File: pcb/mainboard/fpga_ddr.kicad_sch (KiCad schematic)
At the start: 33 parts, among them U12 MT41K64M16TW, U5 XC6SLX16-FTG256

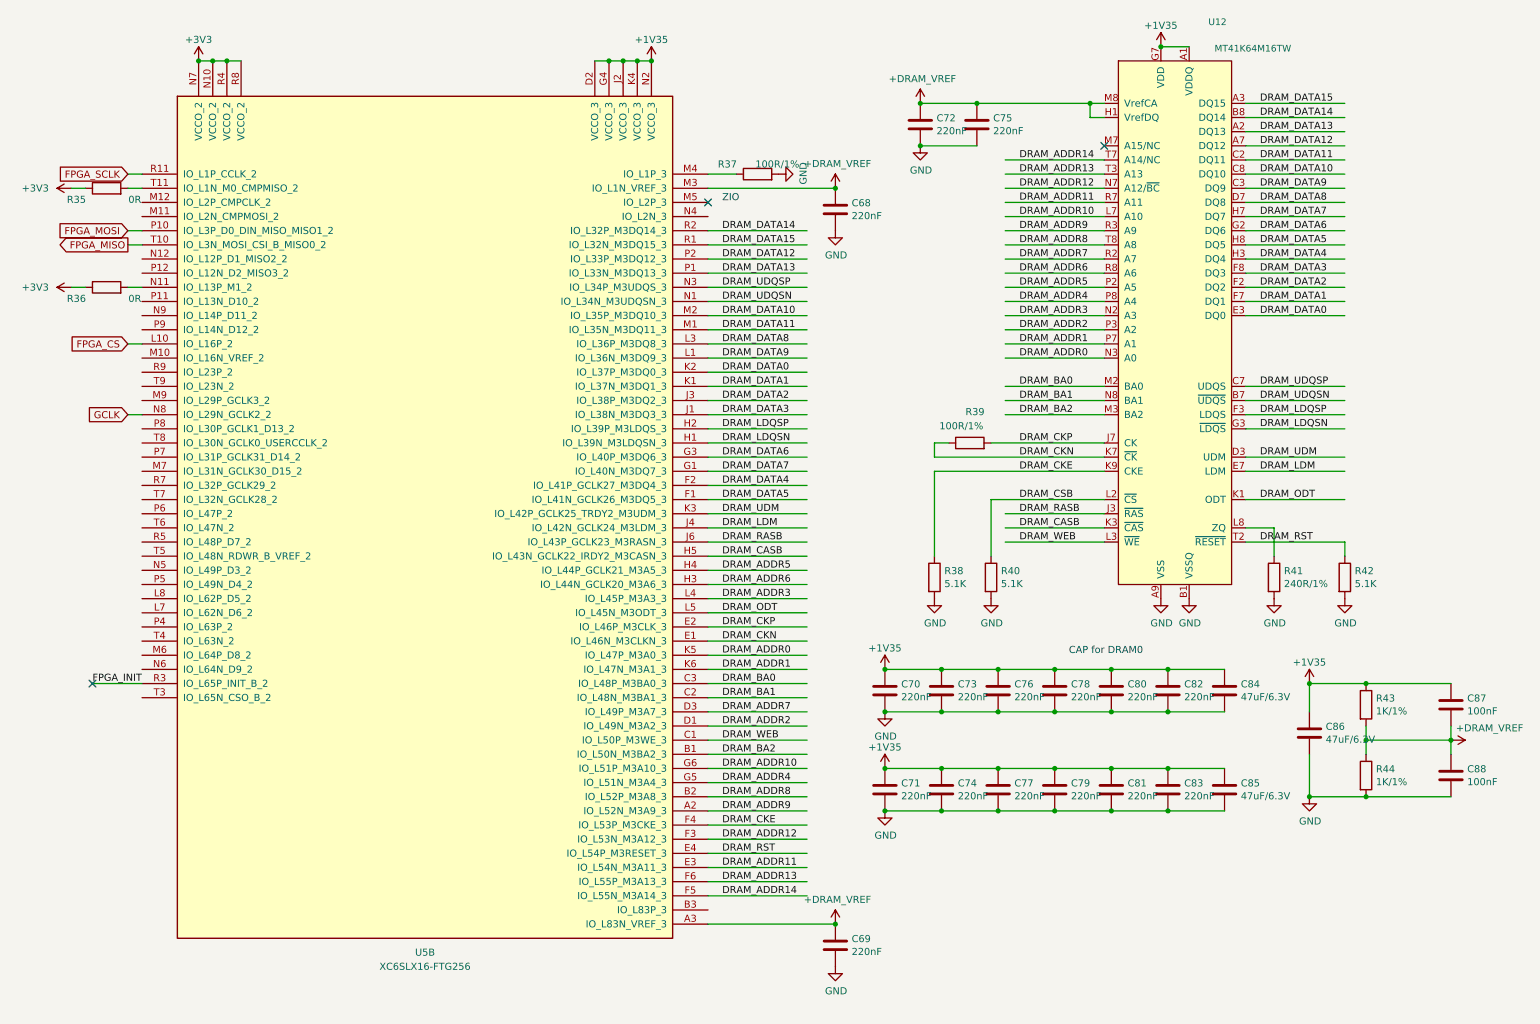
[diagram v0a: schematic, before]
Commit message: PCB r0p9
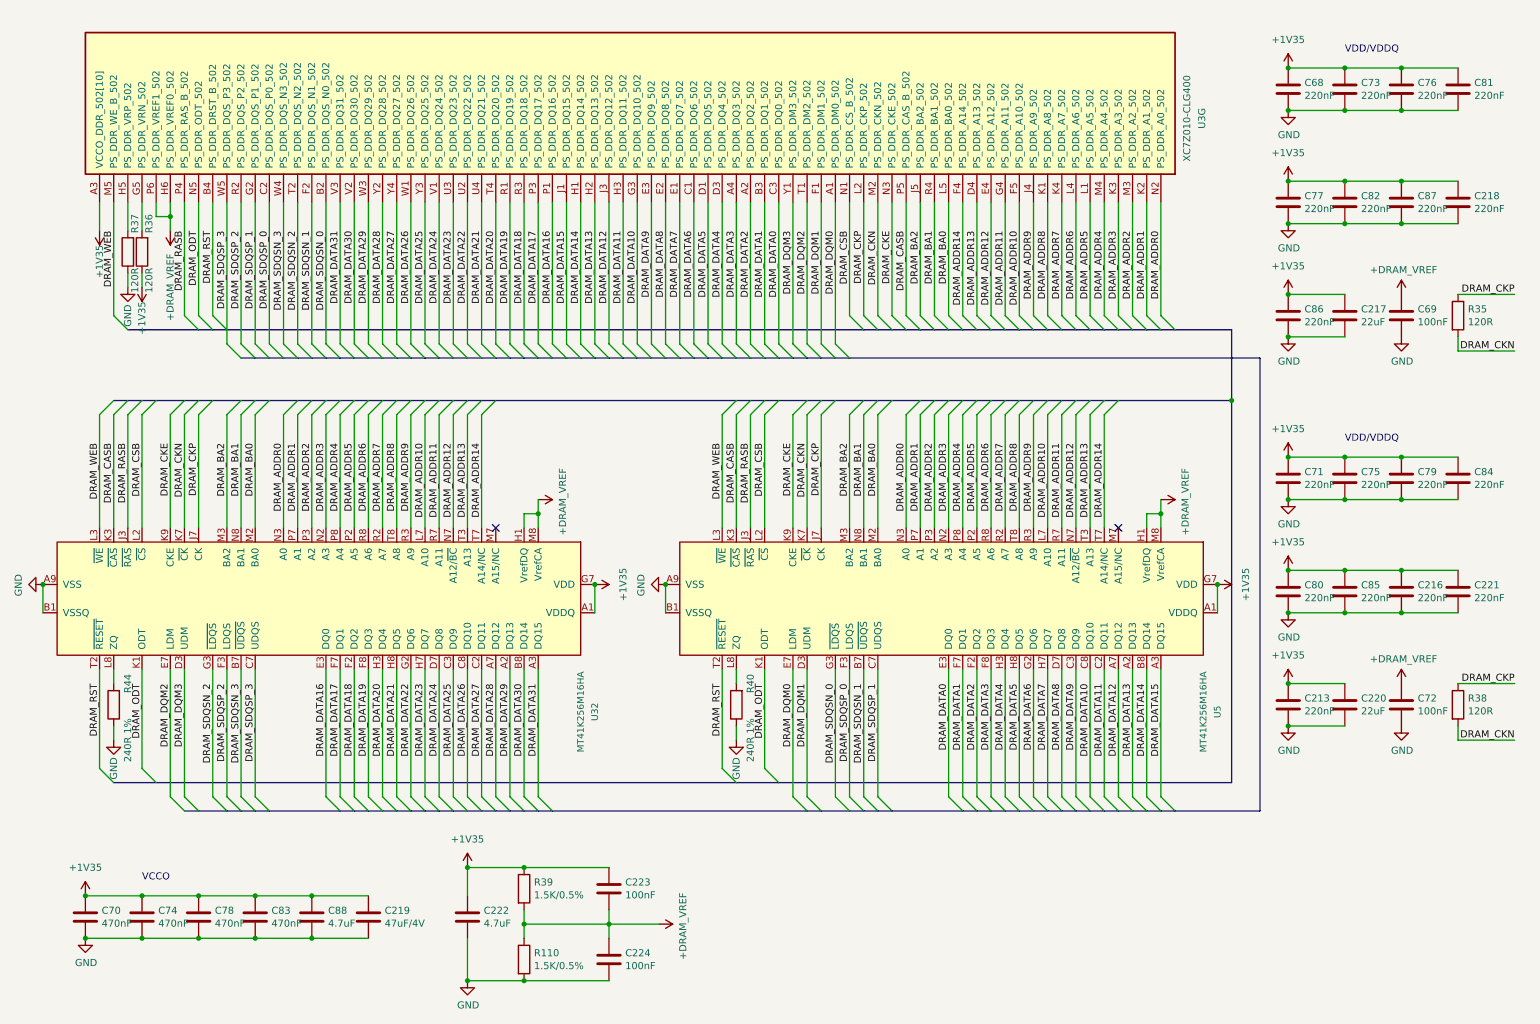
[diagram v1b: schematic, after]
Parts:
- removed R41: 240R/1%, Resistor_SMD:R_0402_1005Metric, symbol Device:R
- removed R42: 5.1K, Resistor_SMD:R_0402_1005Metric, symbol Device:R
- removed R43: 1K/1%, Resistor_SMD:R_0402_1005Metric, symbol Device:R
- removed U12: MT41K64M16TW, footprints:BGA-96_9.0x14.0mm_P0.8mm, symbol symbols:MT41K256M16HA
- removed U5: XC6SLX16-FTG256, footprints:Xilinx_FTG256, symbol FPGA_Xilinx_Spartan6:XC6SLX16-FTG256
- added C213, C216, C218, C221: 220nF, Capacitor_SMD:C_0402_1005Metric, symbol Device:C
- added C217, C220: 22uF, Capacitor_SMD:C_0603_1608Metric, symbol Device:C
- added C219: 47uF/4V, Capacitor_SMD:C_0603_1608Metric, symbol Device:C
- added C222: 4.7uF, Capacitor_SMD:C_0603_1608Metric, symbol Device:C
- added C223, C224: 100nF, Capacitor_SMD:C_0402_1005Metric, symbol Device:C
- added R110: 1.5K/0.5%, Resistor_SMD:R_0402_1005Metric, symbol Device:R
- added U3: XC7Z010-CLG400, Package_BGA:Xilinx_CLG400, symbol symbols:XC7Z007S-CLG400
- added U32, U5: MT41K256M16HA, Package_BGA:BGA-96_9.0x13.0mm_Layout2x3x16_P0.8mm, symbol symbols:MT41K256M16HA
- C68, C71, C73, C75, C76, C77, C79, C80, C81, C82: Ref.Price 0.0036 -> (none)
- C69, C72: value 220nF -> 100nF; Ref.Price 0.0036 -> (none)
- C70, C74, C78, C83: value 220nF -> 470nF; Ref.Price 0.0036 -> (none)
- C84, C85: value 47uF/6.3V -> 220nF; footprint Capacitor_SMD:C_0603_1608Metric -> Capacitor_SMD:C_0402_1005Metric; Ref.Price 0.0301 -> (none)
- C86: value 47uF/6.3V -> 220nF; footprint Capacitor_SMD:C_0603_1608Metric -> Capacitor_SMD:C_0402_1005Metric; Ref.Price 0.0165 -> (none)
- C87: value 100nF -> 220nF; Ref.Price 0.0023 -> (none)
- C88: value 100nF -> 4.7uF; footprint Capacitor_SMD:C_0402_1005Metric -> Capacitor_SMD:C_0603_1608Metric; Ref.Price 0.0023 -> (none)
- R35, R36: value 0R -> 120R; Ref.Price 0.0006 -> (none)
- R37: value 100R/1% -> 120R; Ref.Price 0.0007 -> (none)
- R38: value 5.1K -> 120R; Ref.Price 0.0006 -> (none)
- R39: value 100R/1% -> 1.5K/0.5%; Ref.Price 0.001 -> (none)
- R40: value 5.1K -> 240R 1%; Ref.Price 0.0006 -> (none)
- R44: value 1K/1% -> 240R 1%; Ref.Price 0.0025 -> (none)
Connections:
- net +1V35: now also C68.1, C75.1, C88.1, R36.1, R39.1, C213.1, C216.1, C217.1, C218.1, C219.1, C220.1, C221.1, C222.1, C223.1, U3.A3 (VCCO_DDR_502[10]), U3.D2 (VCCO_DDR_502[10]), U3.E5 (VCCO_DDR_502[10]), U3.G1 (VCCO_DDR_502[10]), U3.H4 (VCCO_DDR_502[10]), U3.L3 (VCCO_DDR_502[10]), U3.P2 (VCCO_DDR_502[10]), U3.R5 (VCCO_DDR_502[10]), U3.U1 (VCCO_DDR_502[10]), U3.V4 (VCCO_DDR_502[10]), U32.A1 (VDDQ), U32.A8 (VDDQ), U32.B2 (VDD), U32.C1 (VDDQ), U32.C9 (VDDQ), U32.D2 (VDDQ), U32.D9 (VDD), U32.E9 (VDDQ), U32.F1 (VDDQ), U32.G7 (VDD), U32.H2 (VDDQ), U32.H9 (VDDQ), U32.K2 (VDD), U32.K8 (VDD), U32.N1 (VDD), U32.N9 (VDD), U32.R1 (VDD), U32.R9 (VDD), U5.A1 (VDDQ), U5.A8 (VDDQ), U5.B2 (VDD), U5.C1 (VDDQ), U5.C9 (VDDQ), U5.D2 (VDDQ), U5.D9 (VDD), U5.E9 (VDDQ), U5.F1 (VDDQ), U5.G7 (VDD), U5.H2 (VDDQ), U5.H9 (VDDQ), U5.K2 (VDD), U5.K8 (VDD), U5.N1 (VDD), U5.N9 (VDD), U5.R1 (VDD), U5.R9 (VDD)
- net +DRAM_VREF: now also R39.2, C223.2, C224.1, R110.1, U3.H6 (PS_DDR_VREF0_502), U3.P6 (PS_DDR_VREF1_502), U32.H1 (VrefDQ), U32.M8 (VrefCA), U5.H1 (VrefDQ), U5.M8 (VrefCA); no longer C68.1, C75.1, C87.2, C88.1, R44.1
- net DRAM_ADDR0: now also U3.N2 (PS_DDR_A0_502), U32.N3 (A0), U5.N3 (A0)
- net DRAM_ADDR1: now also U3.K2 (PS_DDR_A1_502), U32.P7 (A1), U5.P7 (A1)
- net DRAM_ADDR10: now also U3.F5 (PS_DDR_A10_502), U32.L7 (A10), U5.L7 (A10)
- net DRAM_ADDR11: now also U3.G4 (PS_DDR_A11_502), U32.R7 (A11), U5.R7 (A11)
- net DRAM_ADDR12: now also U3.E4 (PS_DDR_A12_502), U32.N7 (A12/~{BC}), U5.N7 (A12/~{BC})
- net DRAM_ADDR13: now also U3.D4 (PS_DDR_A13_502), U32.T3 (A13), U5.T3 (A13)
- net DRAM_ADDR14: now also U3.F4 (PS_DDR_A14_502), U32.T7 (A14/NC), U5.T7 (A14/NC)
- net DRAM_ADDR2: now also U3.M3 (PS_DDR_A2_502), U32.P3 (A2), U5.P3 (A2)
- net DRAM_ADDR3: now also U3.K3 (PS_DDR_A3_502), U32.N2 (A3), U5.N2 (A3)
- net DRAM_ADDR4: now also U3.M4 (PS_DDR_A4_502), U32.P8 (A4), U5.P8 (A4)
- net DRAM_ADDR5: now also U3.L1 (PS_DDR_A5_502), U32.P2 (A5), U5.P2 (A5)
- net DRAM_ADDR6: now also U3.L4 (PS_DDR_A6_502), U32.R8 (A6), U5.R8 (A6)
- net DRAM_ADDR7: now also U3.K4 (PS_DDR_A7_502), U32.R2 (A7), U5.R2 (A7)
- net DRAM_ADDR8: now also U3.K1 (PS_DDR_A8_502), U32.T8 (A8), U5.T8 (A8)
- net DRAM_ADDR9: now also U3.J4 (PS_DDR_A9_502), U32.R3 (A9), U5.R3 (A9)
- net DRAM_BA0: now also U3.L5 (PS_DDR_BA0_502), U32.M2 (BA0), U5.M2 (BA0)
- net DRAM_BA1: now also U3.R4 (PS_DDR_BA1_502), U32.N8 (BA1), U5.N8 (BA1)
- net DRAM_BA2: now also U3.J5 (PS_DDR_BA2_502), U32.M3 (BA2), U5.M3 (BA2)
- net DRAM_CASB: now also U3.P5 (PS_DDR_CAS_B_502), U32.K3 (~{CAS}), U5.K3 (~{CAS})
- net DRAM_CKE: now also U3.N3 (PS_DDR_CKE_502), U32.K9 (CKE), U5.K9 (CKE); no longer R38.1
- net DRAM_CKN: now also R35.2, R38.2, U3.M2 (PS_DDR_CKN_502), U32.K7 (~{CK}), U5.K7 (~{CK}); no longer R39.1
- net DRAM_CKP: now also R35.1, R38.1, U3.L2 (PS_DDR_CKP_502), U32.J7 (CK), U5.J7 (CK); no longer R39.2
- net DRAM_CSB: now also U3.N1 (PS_DDR_CS_B_502), U32.L2 (~{CS}), U5.L2 (~{CS}); no longer R40.1
- net DRAM_DATA0: now also U3.C3 (PS_DDR_DQ0_502), U5.E3 (DQ0)
- net DRAM_DATA1: now also U3.B3 (PS_DDR_DQ1_502), U5.F7 (DQ1)
- net DRAM_DATA10: now also U3.G3 (PS_DDR_DQ10_502), U5.C8 (DQ10)
- net DRAM_DATA11: now also U3.H3 (PS_DDR_DQ11_502), U5.C2 (DQ11)
- net DRAM_DATA12: now also U3.J3 (PS_DDR_DQ12_502), U5.A7 (DQ12)
- net DRAM_DATA13: now also U3.H2 (PS_DDR_DQ13_502), U5.A2 (DQ13)
- net DRAM_DATA14: now also U3.H1 (PS_DDR_DQ14_502), U5.B8 (DQ14)
- net DRAM_DATA15: now also U3.J1 (PS_DDR_DQ15_502), U5.A3 (DQ15)
- net DRAM_DATA2: now also U3.A2 (PS_DDR_DQ2_502), U5.F2 (DQ2)
- net DRAM_DATA3: now also U3.A4 (PS_DDR_DQ3_502), U5.F8 (DQ3)
- net DRAM_DATA4: now also U3.D3 (PS_DDR_DQ4_502), U5.H3 (DQ4)
- net DRAM_DATA5: now also U3.D1 (PS_DDR_DQ5_502), U5.H8 (DQ5)
- net DRAM_DATA6: now also U3.C1 (PS_DDR_DQ6_502), U5.G2 (DQ6)
- net DRAM_DATA7: now also U3.E1 (PS_DDR_DQ7_502), U5.H7 (DQ7)
- net DRAM_DATA8: now also U3.E2 (PS_DDR_DQ8_502), U5.D7 (DQ8)
- net DRAM_DATA9: now also U3.E3 (PS_DDR_DQ9_502), U5.C3 (DQ9)
- net DRAM_ODT: now also U3.N5 (PS_DDR_ODT_502), U32.K1 (ODT), U5.K1 (ODT)
- net DRAM_RASB: now also U3.P4 (PS_DDR_RAS_B_502), U32.J3 (~{RAS}), U5.J3 (~{RAS})
- net DRAM_RST: now also U3.B4 (PS_DDR_DRST_B_502), U32.T2 (~{RESET}), U5.T2 (~{RESET})
- net DRAM_WEB: now also U3.M5 (PS_DDR_WE_B_502), U32.L3 (~{WE}), U5.L3 (~{WE})
- net GND: now also C87.2, R37.1, R40.1, R44.1, C213.2, C216.2, C217.2, C218.2, C219.2, C220.2, C221.2, C222.2, C224.2, R110.2, U32.A9 (VSS), U32.B1 (VSSQ), U32.B3 (VSS), U32.B9 (VSSQ), U32.D1 (VSSQ), U32.D8 (VSSQ), U32.E1 (VSS), U32.E2 (VSSQ), U32.E8 (VSSQ), U32.F9 (VSSQ), U32.G1 (VSSQ), U32.G8 (VSS), U32.G9 (VSSQ), U32.J2 (VSS), U32.J8 (VSS), U32.M1 (VSS), U32.M9 (VSS), U32.P1 (VSS), U32.P9 (VSS), U32.T1 (VSS), U32.T9 (VSS), U5.A9 (VSS), U5.B1 (VSSQ), U5.B3 (VSS), U5.B9 (VSSQ), U5.D1 (VSSQ), U5.D8 (VSSQ), U5.E1 (VSS), U5.E2 (VSSQ), U5.E8 (VSSQ), U5.F9 (VSSQ), U5.G1 (VSSQ), U5.G8 (VSS), U5.G9 (VSSQ), U5.J2 (VSS), U5.J8 (VSS), U5.M1 (VSS), U5.M9 (VSS), U5.P1 (VSS), U5.P9 (VSS), U5.T1 (VSS), U5.T9 (VSS); no longer R37.2, R38.2, R40.2, R44.2
- net at R36.2: now also U3.G5 (PS_DDR_VRN_502)
- removed net +3V3: R35.1, R36.1
- new net: R40.2, U5.L8 (ZQ)
- new net: R37.2, U3.H5 (PS_DDR_VRP_502)
- new net: R44.2, U32.L8 (ZQ)
- new net DRAM_DATA16: U3.P1 (PS_DDR_DQ16_502), U32.E3 (DQ0)
- new net DRAM_DATA17: U3.P3 (PS_DDR_DQ17_502), U32.F7 (DQ1)
- new net DRAM_DATA18: U3.R3 (PS_DDR_DQ18_502), U32.F2 (DQ2)
- new net DRAM_DATA19: U3.R1 (PS_DDR_DQ19_502), U32.F8 (DQ3)
- new net DRAM_DATA20: U3.T4 (PS_DDR_DQ20_502), U32.H3 (DQ4)
- new net DRAM_DATA21: U3.U4 (PS_DDR_DQ21_502), U32.H8 (DQ5)
- new net DRAM_DATA22: U3.U2 (PS_DDR_DQ22_502), U32.G2 (DQ6)
- new net DRAM_DATA23: U3.U3 (PS_DDR_DQ23_502), U32.H7 (DQ7)
- new net DRAM_DATA24: U3.V1 (PS_DDR_DQ24_502), U32.D7 (DQ8)
- new net DRAM_DATA25: U3.Y3 (PS_DDR_DQ25_502), U32.C3 (DQ9)
- new net DRAM_DATA26: U3.W1 (PS_DDR_DQ26_502), U32.C8 (DQ10)
- new net DRAM_DATA27: U3.Y4 (PS_DDR_DQ27_502), U32.C2 (DQ11)
- new net DRAM_DATA28: U3.Y2 (PS_DDR_DQ28_502), U32.A7 (DQ12)
- new net DRAM_DATA29: U3.W3 (PS_DDR_DQ29_502), U32.A2 (DQ13)
- new net DRAM_DATA30: U3.V2 (PS_DDR_DQ30_502), U32.B8 (DQ14)
- new net DRAM_DATA31: U3.V3 (PS_DDR_DQ31_502), U32.A3 (DQ15)
- new net DRAM_DQM0: U3.A1 (PS_DDR_DM0_502), U5.E7 (LDM)
- new net DRAM_DQM1: U3.F1 (PS_DDR_DM1_502), U5.D3 (UDM)
- new net DRAM_DQM2: U3.T1 (PS_DDR_DM2_502), U32.E7 (LDM)
- new net DRAM_DQM3: U3.Y1 (PS_DDR_DM3_502), U32.D3 (UDM)
- new net DRAM_SDQSN_0: U3.B2 (PS_DDR_DQS_N0_502), U5.G3 (~{LDQS})
- new net DRAM_SDQSN_1: U3.F2 (PS_DDR_DQS_N1_502), U5.B7 (~{UDQS})
- new net DRAM_SDQSN_2: U3.T2 (PS_DDR_DQS_N2_502), U32.G3 (~{LDQS})
- new net DRAM_SDQSN_3: U3.W4 (PS_DDR_DQS_N3_502), U32.B7 (~{UDQS})
- new net DRAM_SDQSP_0: U3.C2 (PS_DDR_DQS_P0_502), U5.F3 (LDQS)
- new net DRAM_SDQSP_1: U3.G2 (PS_DDR_DQS_P1_502), U5.C7 (UDQS)
- new net DRAM_SDQSP_2: U3.R2 (PS_DDR_DQS_P2_502), U32.F3 (LDQS)
- new net DRAM_SDQSP_3: U3.W5 (PS_DDR_DQS_P3_502), U32.C7 (UDQS)
- no-connect marks 3 -> 2
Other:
- note added: "VCCO"
- note added: "VDD/VDDQ"
- note removed: "CAP for DRAM0"
- note removed: "ZIO"

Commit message: PCB r0p10 wip
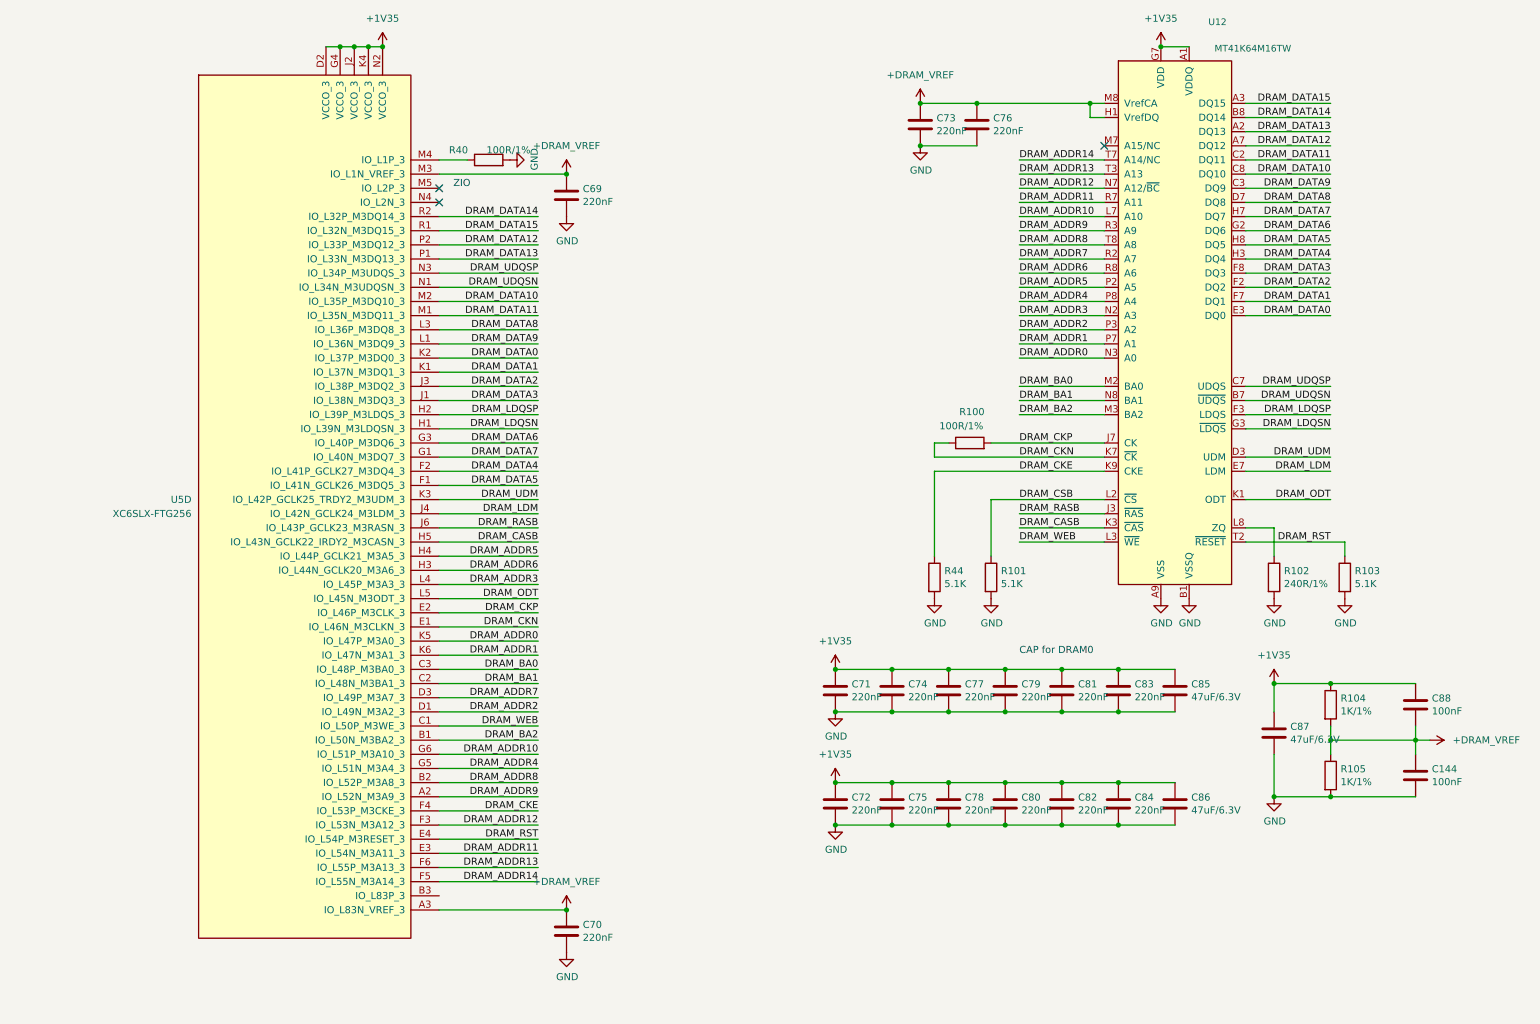
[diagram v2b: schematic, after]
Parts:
- removed C213, C216, C218, C221, C68: 220nF, Capacitor_SMD:C_0402_1005Metric, symbol Device:C
- removed C217, C220: 22uF, Capacitor_SMD:C_0603_1608Metric, symbol Device:C
- removed C219: 47uF/4V, Capacitor_SMD:C_0603_1608Metric, symbol Device:C
- removed C222: 4.7uF, Capacitor_SMD:C_0603_1608Metric, symbol Device:C
- removed C223, C224: 100nF, Capacitor_SMD:C_0402_1005Metric, symbol Device:C
- removed R110, R39: 1.5K/0.5%, Resistor_SMD:R_0402_1005Metric, symbol Device:R
- removed R35, R36, R37, R38: 120R, Resistor_SMD:R_0402_1005Metric, symbol Device:R
- removed U3: XC7Z010-CLG400, Package_BGA:Xilinx_CLG400, symbol symbols:XC7Z007S-CLG400
- removed U32, U5: MT41K256M16HA, Package_BGA:BGA-96_9.0x13.0mm_Layout2x3x16_P0.8mm, symbol symbols:MT41K256M16HA
- added C144: 100nF, Capacitor_SMD:C_0402_1005Metric, symbol Device:C
- added R100: 100R/1%, Resistor_SMD:R_0402_1005Metric, symbol Device:R
- added R101, R103: 5.1K, Resistor_SMD:R_0402_1005Metric, symbol Device:R
- added R102: 240R/1%, Resistor_SMD:R_0402_1005Metric, symbol Device:R
- added R104, R105: 1K/1%, Resistor_SMD:R_0402_1005Metric, symbol Device:R
- added U12: MT41K64M16TW, footprints:BGA-96_9.0x14.0mm_P0.8mm, symbol symbols:MT41K256M16HA
- added U5: XC6SLX-FTG256, symbol symbols:XC6SLX-FTG256
- C69, C72: value 100nF -> 220nF; Ref.Price (none) -> 0.0036
- C70, C74, C78, C83: value 470nF -> 220nF; Ref.Price (none) -> 0.0036
- C71, C73, C75, C76, C77, C79, C80, C81, C82, C84: Ref.Price (none) -> 0.0036
- C85, C86: value 220nF -> 47uF/6.3V; footprint Capacitor_SMD:C_0402_1005Metric -> Capacitor_SMD:C_0603_1608Metric; Ref.Price (none) -> 0.0301
- C87: value 220nF -> 47uF/6.3V; footprint Capacitor_SMD:C_0402_1005Metric -> Capacitor_SMD:C_0603_1608Metric; Ref.Price (none) -> 0.0165
- C88: value 4.7uF -> 100nF; footprint Capacitor_SMD:C_0603_1608Metric -> Capacitor_SMD:C_0402_1005Metric; Ref.Price (none) -> 0.0023
- R40: value 240R 1% -> 100R/1%; Ref.Price (none) -> 0.0007
- R44: value 240R 1% -> 5.1K; Ref.Price (none) -> 0.0006
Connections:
- net +1V35: now also C72.1, R104.1, U12.A1 (VDDQ), U12.A8 (VDDQ), U12.B2 (VDD), U12.C1 (VDDQ), U12.C9 (VDDQ), U12.D2 (VDDQ), U12.D9 (VDD), U12.E9 (VDDQ), U12.F1 (VDDQ), U12.G7 (VDD), U12.H2 (VDDQ), U12.H9 (VDDQ), U12.K2 (VDD), U12.K8 (VDD), U12.N1 (VDD), U12.N9 (VDD), U12.R1 (VDD), U12.R9 (VDD), U5.D2 (VCCO_3), U5.G4 (VCCO_3), U5.J2 (VCCO_3), U5.K4 (VCCO_3), U5.N2 (VCCO_3); no longer C70.1, C73.1, C76.1
- net +DRAM_VREF: now also C70.1, C73.1, C76.1, C88.2, C144.1, R104.2, R105.1, U12.H1 (VrefDQ), U12.M8 (VrefCA), U5.A3 (IO_L83N_VREF_3), U5.M3 (IO_L1N_VREF_3); no longer C72.1
- net DRAM_ADDR0: now also U12.N3 (A0), U5.K5 (IO_L47P_M3A0_3)
- net DRAM_ADDR1: now also U12.P7 (A1), U5.K6 (IO_L47N_M3A1_3)
- net DRAM_ADDR10: now also U12.L7 (A10), U5.G6 (IO_L51P_M3A10_3)
- net DRAM_ADDR11: now also U12.R7 (A11), U5.E3 (IO_L54N_M3A11_3)
- net DRAM_ADDR12: now also U12.N7 (A12/~{BC}), U5.F3 (IO_L53N_M3A12_3)
- net DRAM_ADDR13: now also U12.T3 (A13), U5.F6 (IO_L55P_M3A13_3)
- net DRAM_ADDR14: now also U12.T7 (A14/NC), U5.F5 (IO_L55N_M3A14_3)
- net DRAM_ADDR2: now also U12.P3 (A2), U5.D1 (IO_L49N_M3A2_3)
- net DRAM_ADDR3: now also U12.N2 (A3), U5.L4 (IO_L45P_M3A3_3)
- net DRAM_ADDR4: now also U12.P8 (A4), U5.G5 (IO_L51N_M3A4_3)
- net DRAM_ADDR5: now also U12.P2 (A5), U5.H4 (IO_L44P_GCLK21_M3A5_3)
- net DRAM_ADDR6: now also U12.R8 (A6), U5.H3 (IO_L44N_GCLK20_M3A6_3)
- net DRAM_ADDR7: now also U12.R2 (A7), U5.D3 (IO_L49P_M3A7_3)
- net DRAM_ADDR8: now also U12.T8 (A8), U5.B2 (IO_L52P_M3A8_3)
- net DRAM_ADDR9: now also U12.R3 (A9), U5.A2 (IO_L52N_M3A9_3)
- net DRAM_BA0: now also U12.M2 (BA0), U5.C3 (IO_L48P_M3BA0_3)
- net DRAM_BA1: now also U12.N8 (BA1), U5.C2 (IO_L48N_M3BA1_3)
- net DRAM_BA2: now also U12.M3 (BA2), U5.B1 (IO_L50N_M3BA2_3)
- net DRAM_CASB: now also U12.K3 (~{CAS}), U5.H5 (IO_L43N_GCLK22_IRDY2_M3CASN_3)
- net DRAM_CKE: now also R44.1, U12.K9 (CKE), U5.F4 (IO_L53P_M3CKE_3)
- net DRAM_CKN: now also R100.1, U12.K7 (~{CK}), U5.E1 (IO_L46N_M3CLKN_3)
- net DRAM_CKP: now also R100.2, U12.J7 (CK), U5.E2 (IO_L46P_M3CLK_3)
- net DRAM_CSB: now also R101.1, U12.L2 (~{CS})
- net DRAM_DATA0: now also U12.E3 (DQ0), U5.K2 (IO_L37P_M3DQ0_3)
- net DRAM_DATA1: now also U12.F7 (DQ1), U5.K1 (IO_L37N_M3DQ1_3)
- net DRAM_DATA10: now also U12.C8 (DQ10), U5.M2 (IO_L35P_M3DQ10_3)
- net DRAM_DATA11: now also U12.C2 (DQ11), U5.M1 (IO_L35N_M3DQ11_3)
- net DRAM_DATA12: now also U12.A7 (DQ12), U5.P2 (IO_L33P_M3DQ12_3)
- net DRAM_DATA13: now also U12.A2 (DQ13), U5.P1 (IO_L33N_M3DQ13_3)
- net DRAM_DATA14: now also U12.B8 (DQ14), U5.R2 (IO_L32P_M3DQ14_3)
- net DRAM_DATA15: now also U12.A3 (DQ15), U5.R1 (IO_L32N_M3DQ15_3)
- net DRAM_DATA2: now also U12.F2 (DQ2), U5.J3 (IO_L38P_M3DQ2_3)
- net DRAM_DATA3: now also U12.F8 (DQ3), U5.J1 (IO_L38N_M3DQ3_3)
- net DRAM_DATA4: now also U12.H3 (DQ4), U5.F2 (IO_L41P_GCLK27_M3DQ4_3)
- net DRAM_DATA5: now also U12.H8 (DQ5), U5.F1 (IO_L41N_GCLK26_M3DQ5_3)
- net DRAM_DATA6: now also U12.G2 (DQ6), U5.G3 (IO_L40P_M3DQ6_3)
- net DRAM_DATA7: now also U12.H7 (DQ7), U5.G1 (IO_L40N_M3DQ7_3)
- net DRAM_DATA8: now also U12.D7 (DQ8), U5.L3 (IO_L36P_M3DQ8_3)
- net DRAM_DATA9: now also U12.C3 (DQ9), U5.L1 (IO_L36N_M3DQ9_3)
- net DRAM_ODT: now also U12.K1 (ODT), U5.L5 (IO_L45N_M3ODT_3)
- net DRAM_RASB: now also U12.J3 (~{RAS}), U5.J6 (IO_L43P_GCLK23_M3RASN_3)
- net DRAM_RST: now also R103.1, U12.T2 (~{RESET}), U5.E4 (IO_L54P_M3RESET_3)
- net DRAM_WEB: now also U12.L3 (~{WE}), U5.C1 (IO_L50P_M3WE_3)
- net GND: now also R40.2, R44.2, C144.2, R101.2, R102.2, R103.2, R105.2, U12.A9 (VSS), U12.B1 (VSSQ), U12.B3 (VSS), U12.B9 (VSSQ), U12.D1 (VSSQ), U12.D8 (VSSQ), U12.E1 (VSS), U12.E2 (VSSQ), U12.E8 (VSSQ), U12.F9 (VSSQ), U12.G1 (VSSQ), U12.G8 (VSS), U12.G9 (VSSQ), U12.J1 (VSS), U12.J2 (VSS), U12.J8 (VSS), U12.J9 (VSS), U12.L1 (VSS), U12.L9 (VSS), U12.M1 (VSS), U12.M9 (VSS), U12.P1 (VSS), U12.P9 (VSS), U12.T1 (VSS), U12.T9 (VSS); no longer C88.2, R40.1, R44.1
- new net: R102.1, U12.L8 (ZQ)
- new net: R40.1, U5.M4 (IO_L1P_3)
- new net DRAM_LDM: U12.E7 (LDM), U5.J4 (IO_L42N_GCLK24_M3LDM_3)
- new net DRAM_LDQSN: U12.G3 (~{LDQS}), U5.H1 (IO_L39N_M3LDQSN_3)
- new net DRAM_LDQSP: U12.F3 (LDQS), U5.H2 (IO_L39P_M3LDQS_3)
- new net DRAM_UDM: U12.D3 (UDM), U5.K3 (IO_L42P_GCLK25_TRDY2_M3UDM_3)
- new net DRAM_UDQSN: U12.B7 (~{UDQS}), U5.N1 (IO_L34N_M3UDQSN_3)
- new net DRAM_UDQSP: U12.C7 (UDQS), U5.N3 (IO_L34P_M3UDQS_3)
- no-connect marks 2 -> 3
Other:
- note added: "CAP for DRAM0"
- note added: "ZIO"
- note removed: "VCCO"
- note removed: "VDD/VDDQ"
